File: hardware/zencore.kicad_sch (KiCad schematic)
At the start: 34 parts, among them J1 Micro_SD_Card, J2 USB_C_Receptacle_USB2.0_16P, J3 Conn_01x20_Pin, J4 Conn_01x20_Pin, SW1 SW_Push, SW2 SW_Push, U1 W25Q128JVS, U2 STM32F411CEUx, U3 TPS62162DSG, Y1 Crystal_GND24_Small

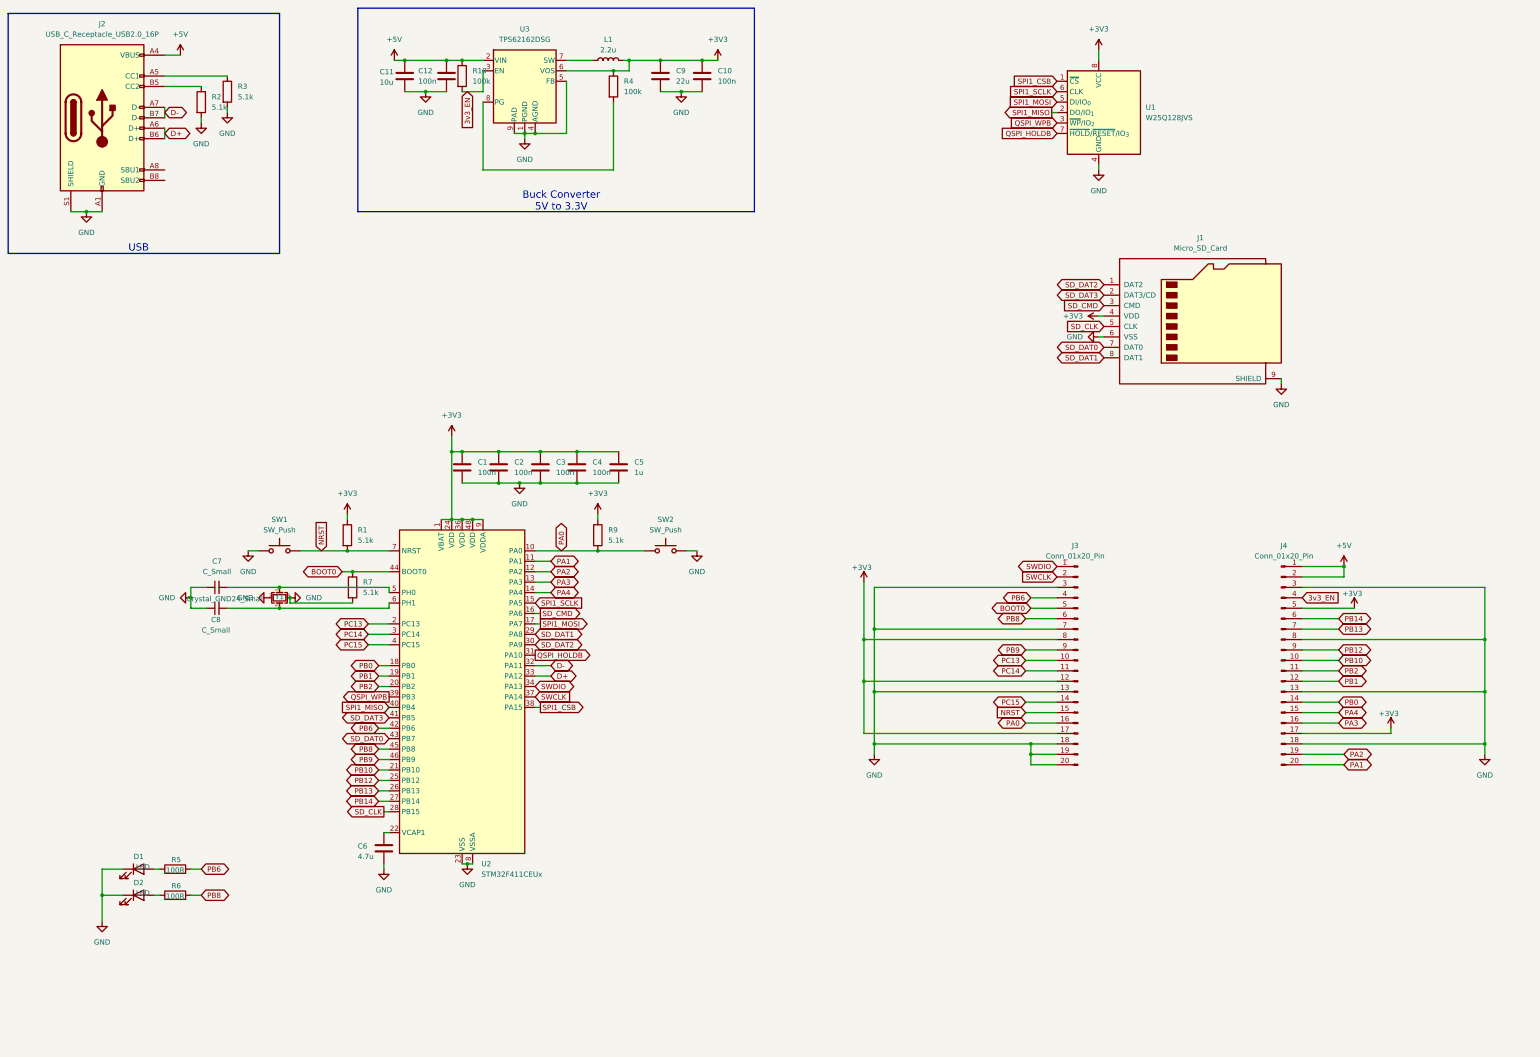
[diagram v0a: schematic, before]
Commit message: PCB production files added
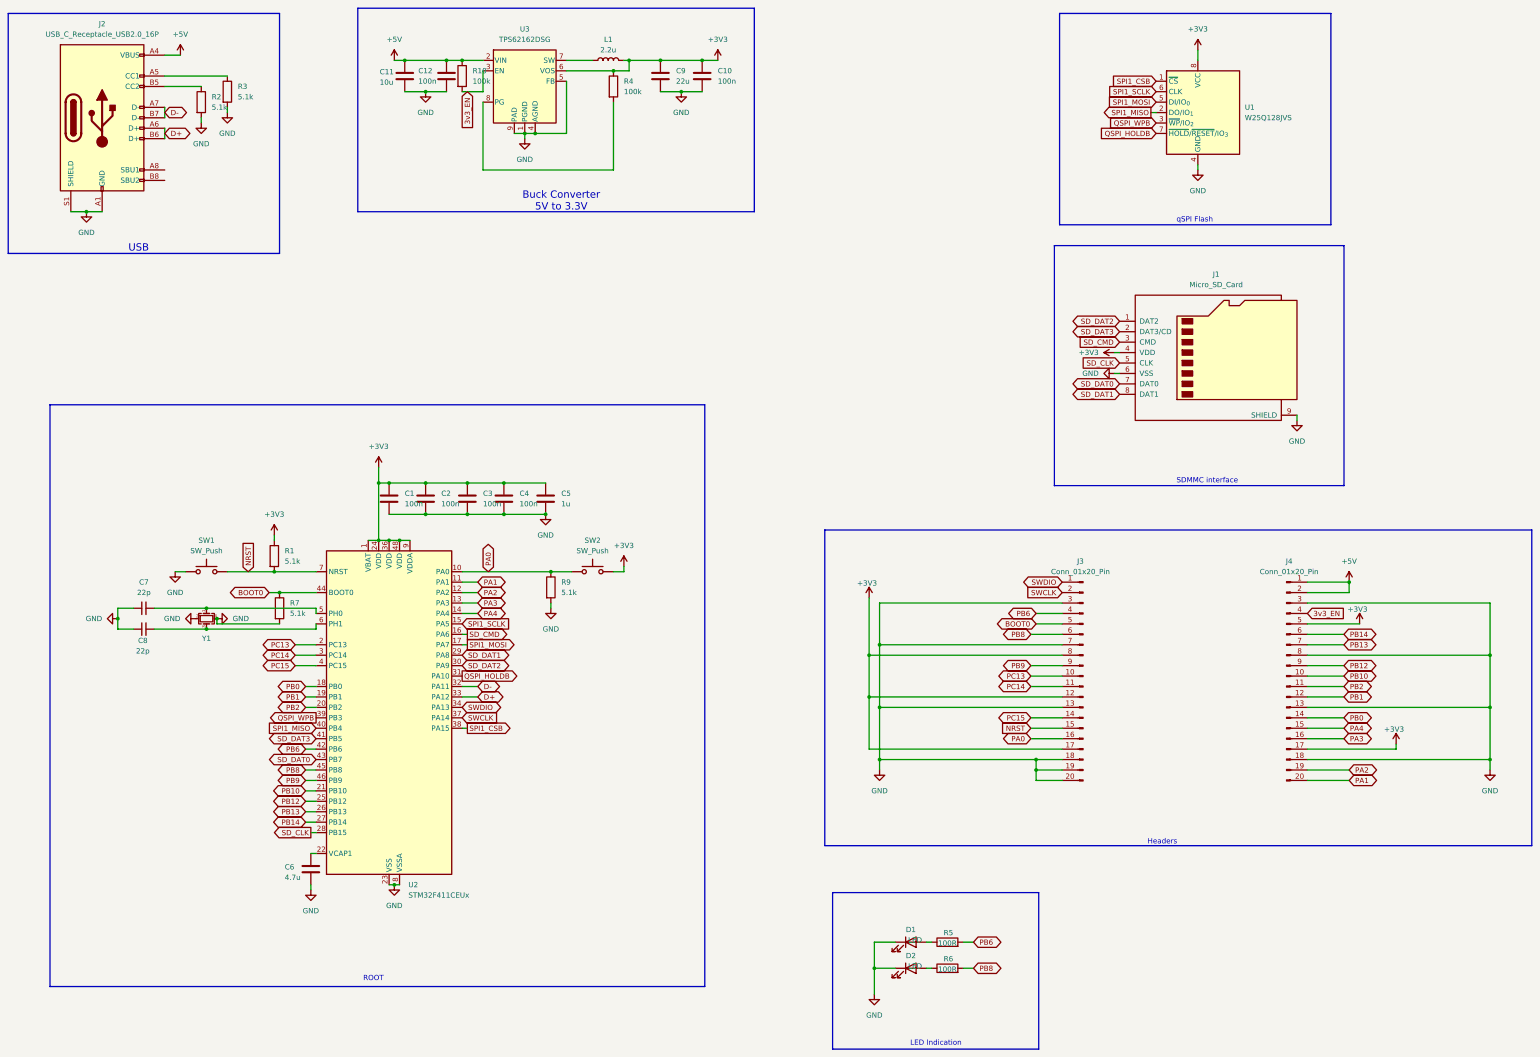
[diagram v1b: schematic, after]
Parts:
- C7, C8: value C_Small -> 22p
- L1: footprint Inductor_SMD:L_0603_1608Metric -> Inductor_SMD:L_0805_2012Metric
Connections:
- net +3V3: now also SW2.2; no longer R9.1
- net GND: now also R9.2; no longer SW2.2
- net PA0: now also R9.1; no longer R9.2
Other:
- note added: "Headers"
- note added: "LED Indication"
- note added: "ROOT"
- note added: "SDMMC interface"
- note added: "qSPI Flash"
- title: (none) -> ZenCore
- moved on the sheet: C1, C2, C3, C4, C5, C6, C7, C8, D1, D2, J1, J3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
